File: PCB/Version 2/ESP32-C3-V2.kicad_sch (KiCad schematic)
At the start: 33 parts, among them J2 DPS_PPS_Right_Angle, J3 HCZZ0001-4, SW1 TS-1187A-B-A-B, SW2 TS-1187A-B-A-B, U1 USB-C-16P-SMD, U3 ESP32-C3, Y1 40MHz_S3240000151040

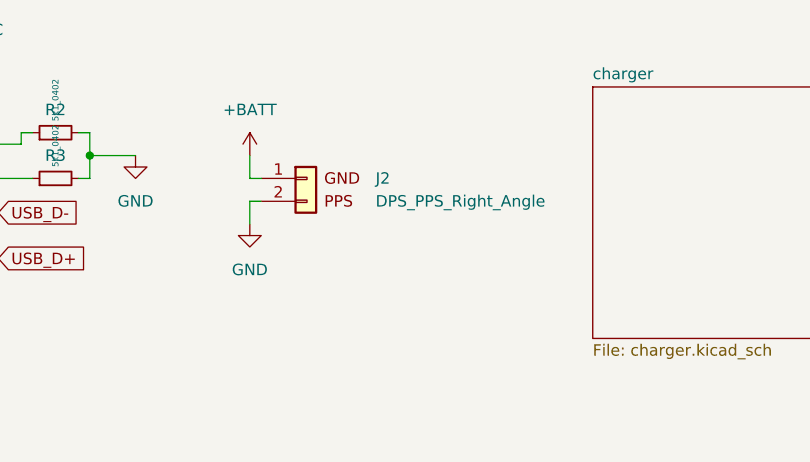
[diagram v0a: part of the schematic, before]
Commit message: update
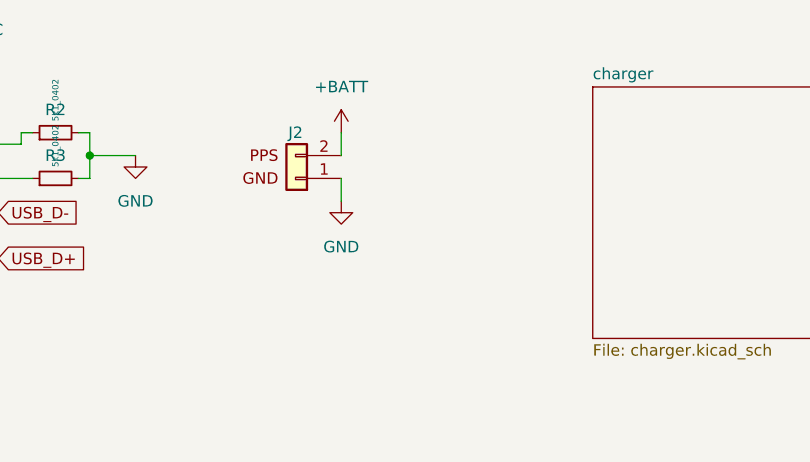
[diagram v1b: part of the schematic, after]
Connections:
- net +BATT: now also J2.2 (Pin_2); no longer J2.1 (Pin_1)
- net GND: now also J2.1 (Pin_1); no longer J2.2 (Pin_2)
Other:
- moved on the sheet: J2
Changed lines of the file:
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@@
 	(wire
 		(pts
-			(xy 76.2 34.29) (xy 74.93 34.29)
-		)
-		(stroke
-			(width 0)
-			(type default)
-		)
-	)
-	(wire
-		(pts
 			(xy 132.08 135.89) (xy 133.35 135.89)
 		)
@@
 	(wire
 		(pts
-			(xy 74.93 31.75) (xy 74.93 34.29)
+			(xy 85.09 29.21) (xy 85.09 31.75)
 		)
 		(stroke
@@
 	(wire
 		(pts
-			(xy 74.93 36.83) (xy 76.2 36.83)
-		)
-		(stroke
-			(width 0)
-			(type default)
-		)
-	)
-	(wire
-		(pts
 			(xy 45.72 43.18) (xy 46.99 43.18)
 		)
@@
 	(wire
 		(pts
-			(xy 74.93 39.37) (xy 74.93 36.83)
+			(xy 85.09 36.83) (xy 85.09 34.29)
 		)
 		(stroke
@@
 	(symbol
 		(lib_id "power:GND")
-		(at 74.93 39.37 0)
+		(at 85.09 36.83 0)
 		(unit 1)
 		(exclude_from_sim no)
@@
 		(fields_autoplaced yes)
 		(property "Reference" "#PWR06"
-			(at 74.93 45.72 0)
+			(at 85.09 43.18 0)
 			(effects
 				(font
@@
 		)
 		(property "Value" "GND"
-			(at 74.93 44.45 0)
+			(at 85.09 41.91 0)
 			(effects
 				(font
@@
 		)
 		(property "Footprint" ""
-			(at 74.93 39.37 0)
+			(at 85.09 36.83 0)
 			(effects
 				(font
@@
 		)
 		(property "Datasheet" ""
-			(at 74.93 39.37 0)
+			(at 85.09 36.83 0)
 			(effects
 				(font
@@
 		)
 		(property "Description" ""
-			(at 74.93 39.37 0)
+			(at 85.09 36.83 0)
 			(effects
 				(font
@@
 	(symbol
 		(lib_id "DPS_connectors:DPS_PPS_Right_Angle")
-		(at 81.28 35.56 0)
+		(at 80.01 33.02 180)
 		(unit 1)
 		(exclude_from_sim no)
@@
 		(on_board yes)
 		(dnp no)
-		(fields_autoplaced yes)
 		(property "Reference" "J2"
-			(at 88.9 34.29 0)
+			(at 80.01 29.21 0)
 			(effects
 				(font
 					(size 1.27 1.27)
 				)
-				(justify left)
 			)
 		)
 		(property "Value" "DPS_PPS_Right_Angle"
-			(at 88.9 36.83 0)
+			(at 72.39 28.194 0)
 			(effects
 				(font
 					(size 1.27 1.27)
 				)
-				(justify left)
+				(hide yes)
 			)
 		)
 		(property "Footprint" "Connector_JST:JST_PH_S2B-PH-K_1x02_P2.00mm_Horizontal"
-			(at 81.28 36.83 0)
+			(at 80.01 31.75 0)
 			(effects
 				(font
@@
 		)
 		(property "Datasheet" "https://datasheet.lcsc.com/lcsc/2303231100_SHOU-HAN-2-0mm-2P-WZ_C5368738.pdf"
-			(at 81.28 36.83 0)
+			(at 80.01 31.75 0)
 			(effects
 				(font
@@
 		)
 		(property "Description" ""
-			(at 81.28 35.56 0)
+			(at 80.01 33.02 0)
 			(effects
 				(font
@@
 		)
 		(property "LCSC" "C7465576"
-			(at 81.28 36.83 0)
+			(at 80.01 31.75 0)
 			(effects
 				(font
@@
 	(symbol
 		(lib_id "power:+BATT")
-		(at 74.93 31.75 0)
+		(at 85.09 29.21 0)
 		(unit 1)
 		(exclude_from_sim no)
@@
 		(fields_autoplaced yes)
 		(property "Reference" "#PWR010"
-			(at 74.93 35.56 0)
+			(at 85.09 33.02 0)
 			(effects
 				(font
@@
 		)
 		(property "Value" "+BATT"
-			(at 74.93 26.67 0)
+			(at 85.09 24.13 0)
 			(effects
 				(font
@@
 		)
 		(property "Footprint" ""
-			(at 74.93 31.75 0)
+			(at 85.09 29.21 0)
 			(effects
 				(font
@@
 		)
 		(property "Datasheet" ""
-			(at 74.93 31.75 0)
+			(at 85.09 29.21 0)
 			(effects
 				(font
@@
 		)
 		(property "Description" ""
-			(at 74.93 31.75 0)
+			(at 85.09 29.21 0)
 			(effects
 				(font

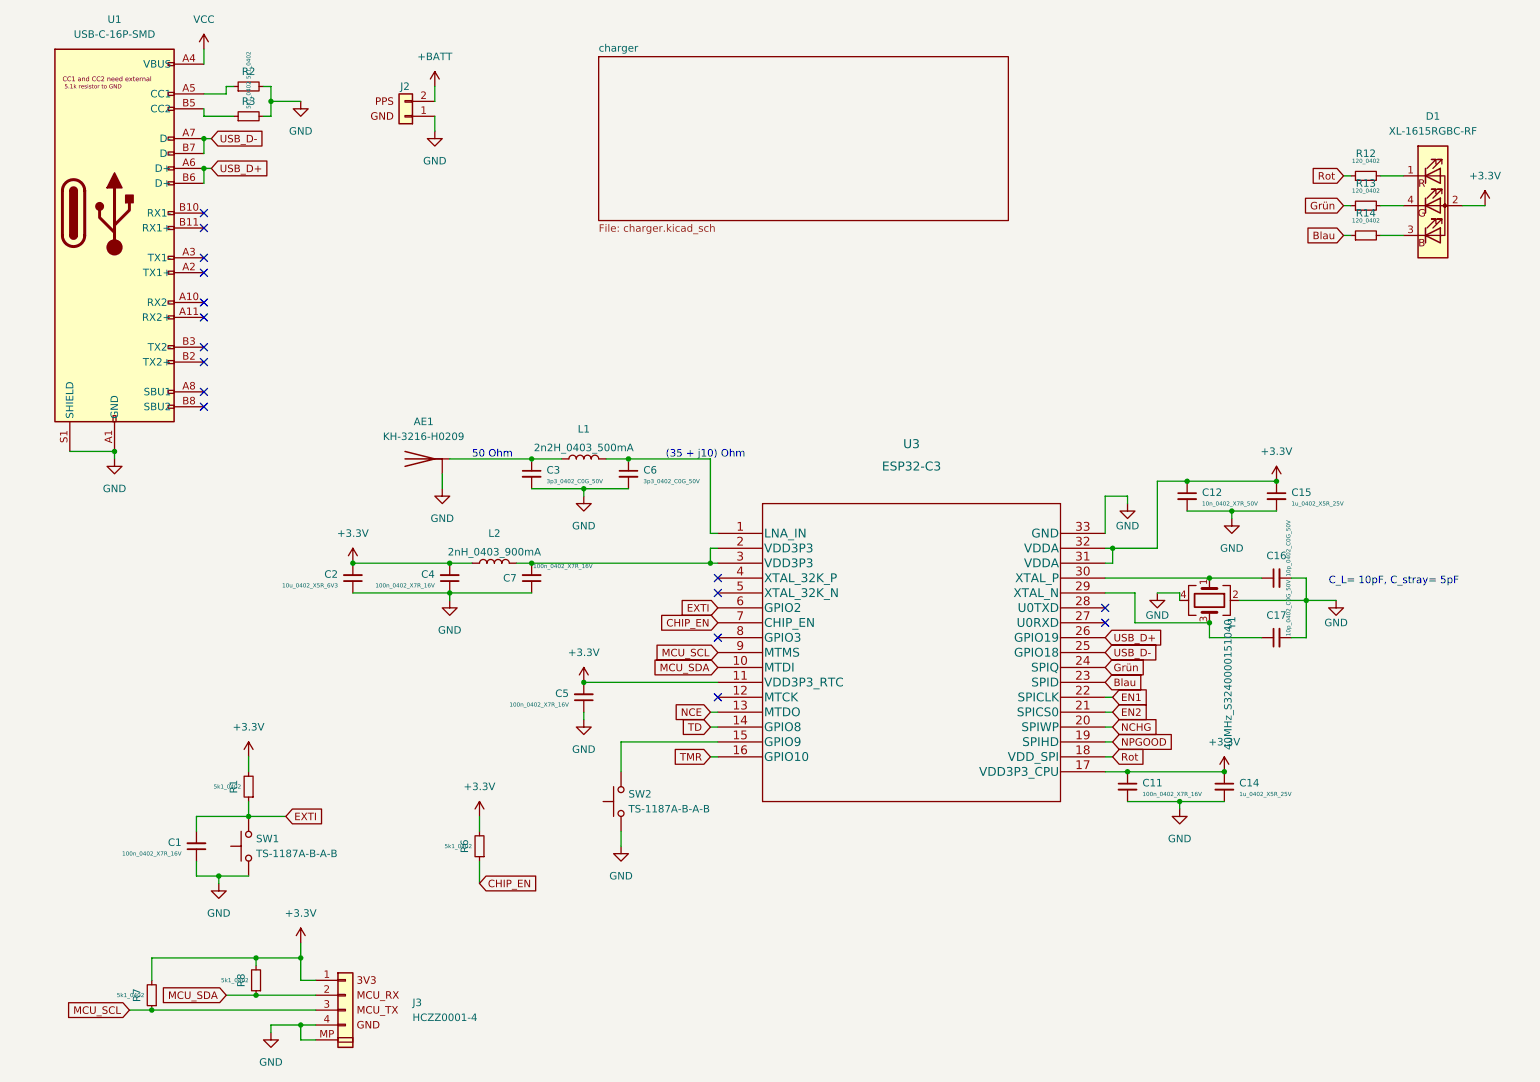
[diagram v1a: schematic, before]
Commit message: Working on Version 2
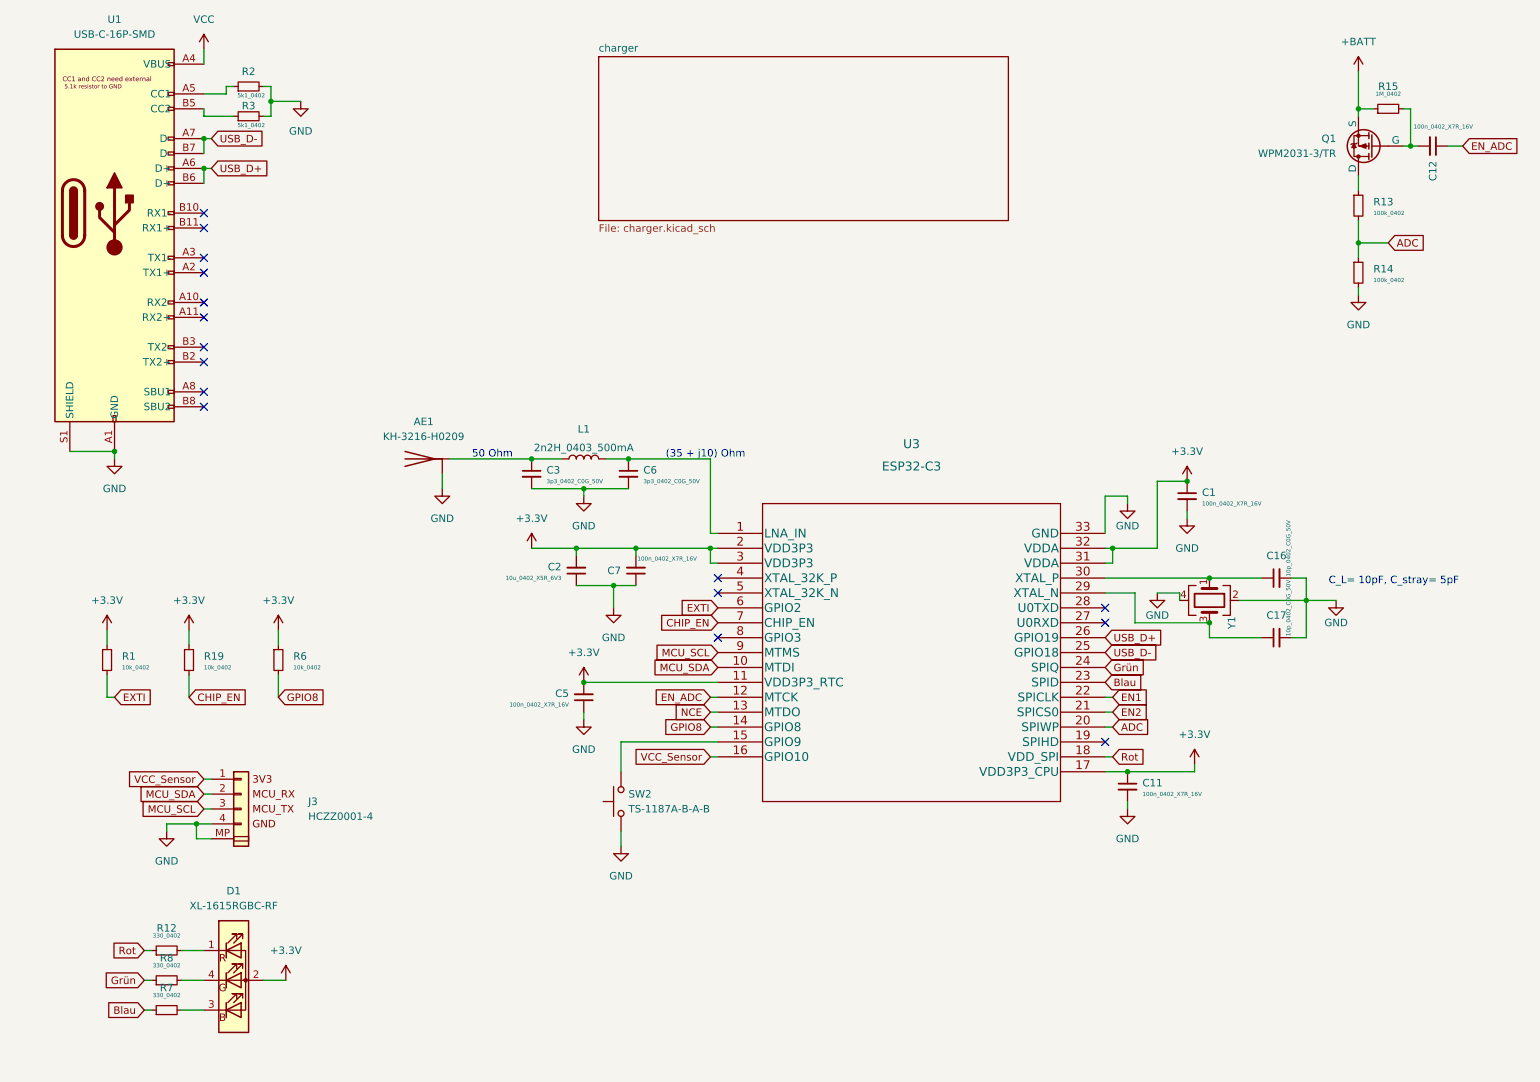
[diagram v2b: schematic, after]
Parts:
- removed C12: 10n_0402_X7R_50V, Capacitor_SMD:C_0402_1005Metric, symbol capacitor_smd_standard:10n_0402_X7R_50V
- removed C14, C15: 1u_0402_X5R_25V, Capacitor_SMD:C_0402_1005Metric, symbol capacitor_smd_standard:1u_0402_X5R_25V
- removed C4: 100n_0402_X7R_16V, Capacitor_SMD:C_0402_1005Metric, symbol capacitor_smd_standard:100n_0402_X7R_16V
- removed J2: DPS_PPS_Right_Angle, Connector_JST:JST_PH_S2B-PH-K_1x02_P2.00mm_Horizontal, symbol DPS_connectors:DPS_PPS_Right_Angle
- removed L2: 2nH_0403_900mA, Resistor_SMD:R_0402_1005Metric, symbol ESP32-C3_Bib:2nH_0403_900mA
- removed R1, R6, R7, R8: 5k1_0402, Resistor_SMD:R_0402_1005Metric, symbol resistor_smd_standard:5k1_0402
- removed R12, R13, R14: 120_0402, Resistor_SMD:R_0402_1005Metric, symbol resistor_smd_standard:120_0402
- removed SW1: TS-1187A-B-A-B, switch:SW_SPST_TL3305B, symbol 1_switch:TS-1187A-B-A-B
- added C12: 100n_0402_X7R_16V, Capacitor_SMD:C_0402_1005Metric, symbol capacitor_smd_standard:100n_0402_X7R_16V
- added Q1: WPM2031-3/TR, Package_TO_SOT_SMD:SOT-723, symbol Lil-Lib:PMOS
- added R1, R19, R6: 10k_0402, Resistor_SMD:R_0402_1005Metric, symbol resistor_smd_standard:10k_0402
- added R12, R7, R8: 330_0402, Resistor_SMD:R_0402_1005Metric, symbol resistor_smd_standard:330_0402
- added R13, R14: 100k_0402, Resistor_SMD:R_0402_1005Metric, symbol resistor_smd_standard:100k_0402
- added R15: 1M_0402, Resistor_SMD:R_0402_1005Metric, symbol resistor_smd_standard:1M_0402
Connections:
- net +3.3V: now also C1.1, C7.2, U3.2 (VDD3P3), U3.3 (VDD3P3), R1.1, R19.1, R6.1; no longer J3.1 (Pin_1)
- net +BATT: now also Q1.2 (S), R15.1
- net Blau: now also R7.1
- net CHIP_EN: now also R19.2
- net EXTI: now also R1.2; no longer C1.2
- net GND: now also C1.2, R14.2; no longer C1.1
- net Grün: now also R8.1
- net Rot: now also R12.1
- net at D1.1 (RK): now also R12.2
- net at D1.3 (BK): now also R7.2
- net at D1.4 (GK): now also R8.2
- net EN_ADC: now reaches U3.12 (MTCK)
- net EN_ADC: now also C12.1
- net NCHG renamed ADC
- net ADC: now also R13.2, R14.1
- net NPGOOD: no longer names the net of U3.19 (SPIHD)
- net TD renamed GPIO8
- net GPIO8: now also R6.2
- net TMR renamed VCC_Sensor
- net VCC_Sensor: now also J3.1 (Pin_1)
- new net: C12.2, Q1.1 (G), R15.2
- new net: Q1.3 (D), R13.1
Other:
- moved on the sheet: C2, C7, D1

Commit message: Version 2
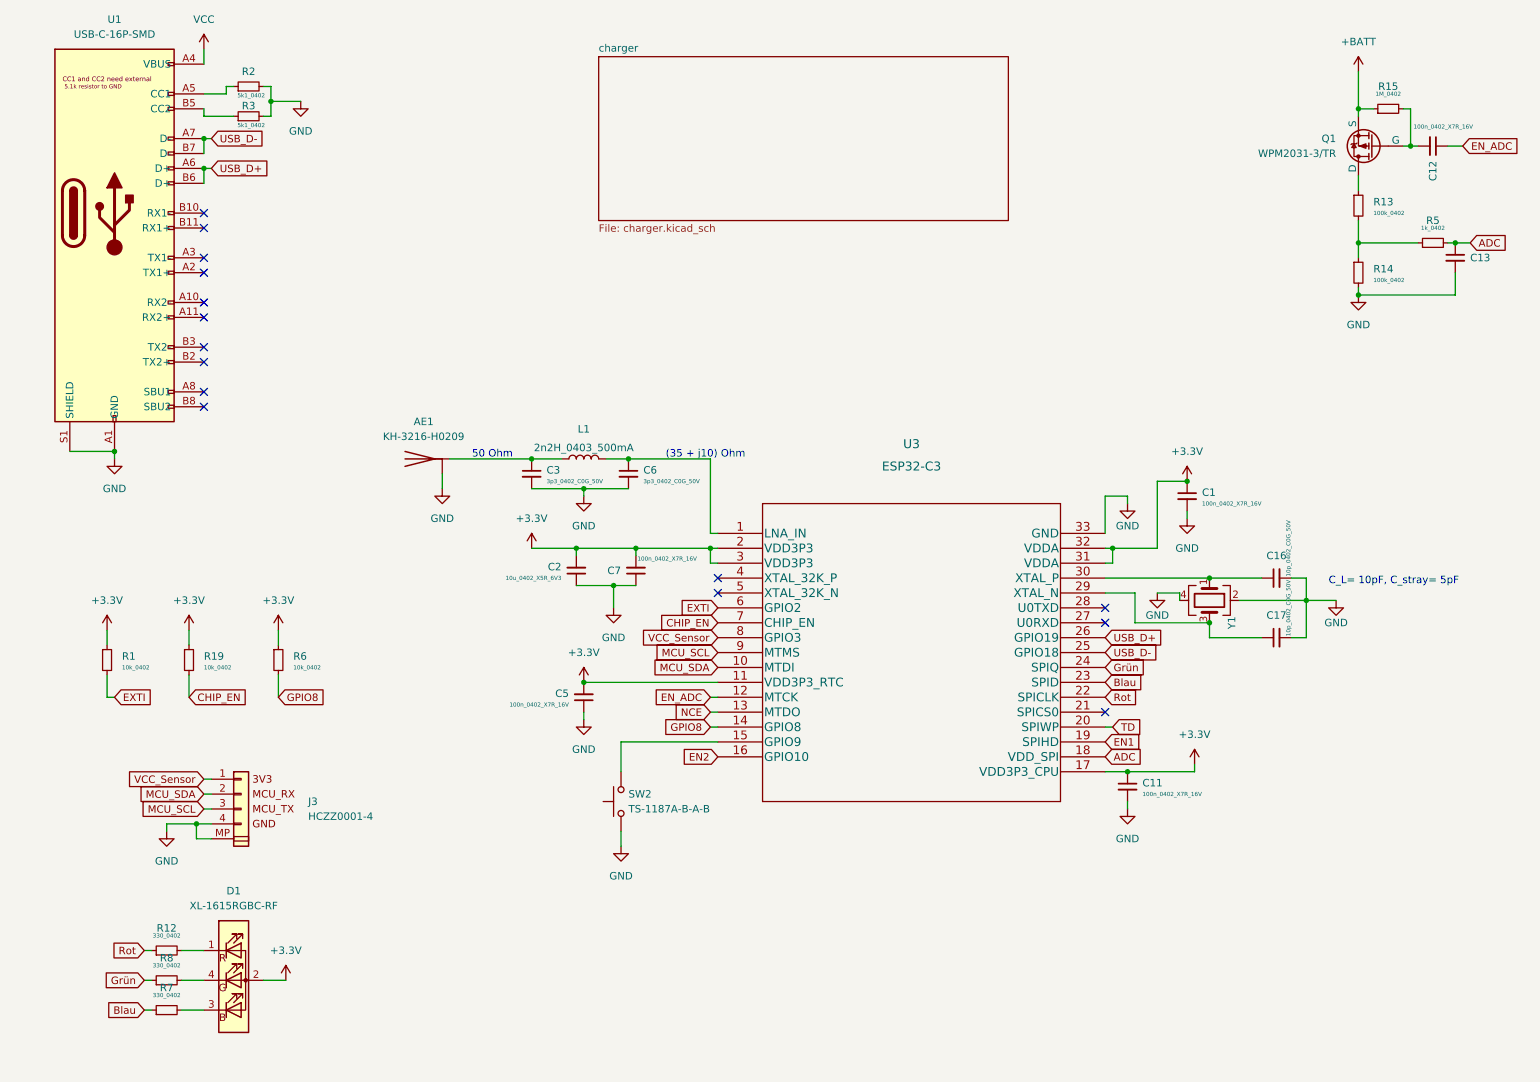
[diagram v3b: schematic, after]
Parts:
- added C13: 100n_0402_X7R_16V, Capacitor_SMD:C_0402_1005Metric, symbol capacitor_smd_standard:100n_0402_X7R_16V
- added R5: 1k_0402, Resistor_SMD:R_0402_1005Metric, symbol resistor_smd_standard:1k_0402
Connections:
- net ADC: now also U3.18 (VDD_SPI), C13.1, R5.2; no longer R13.2, R14.1, U3.20 (SPIWP)
- net EN1: now also U3.19 (SPIHD); no longer U3.22 (SPICLK)
- net EN2: now also U3.16 (GPIO10); no longer U3.21 (SPICS0)
- net GND: now also C13.2
- net Rot: now also U3.22 (SPICLK); no longer U3.18 (VDD_SPI)
- net VCC_Sensor: now also U3.8 (GPIO3); no longer U3.16 (GPIO10)
- new net: R13.2, R14.1, R5.1
- new net TD: U3.20 (SPIWP)
- no-connect marks 16 -> 15

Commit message: V2 für Kontrolle fertig
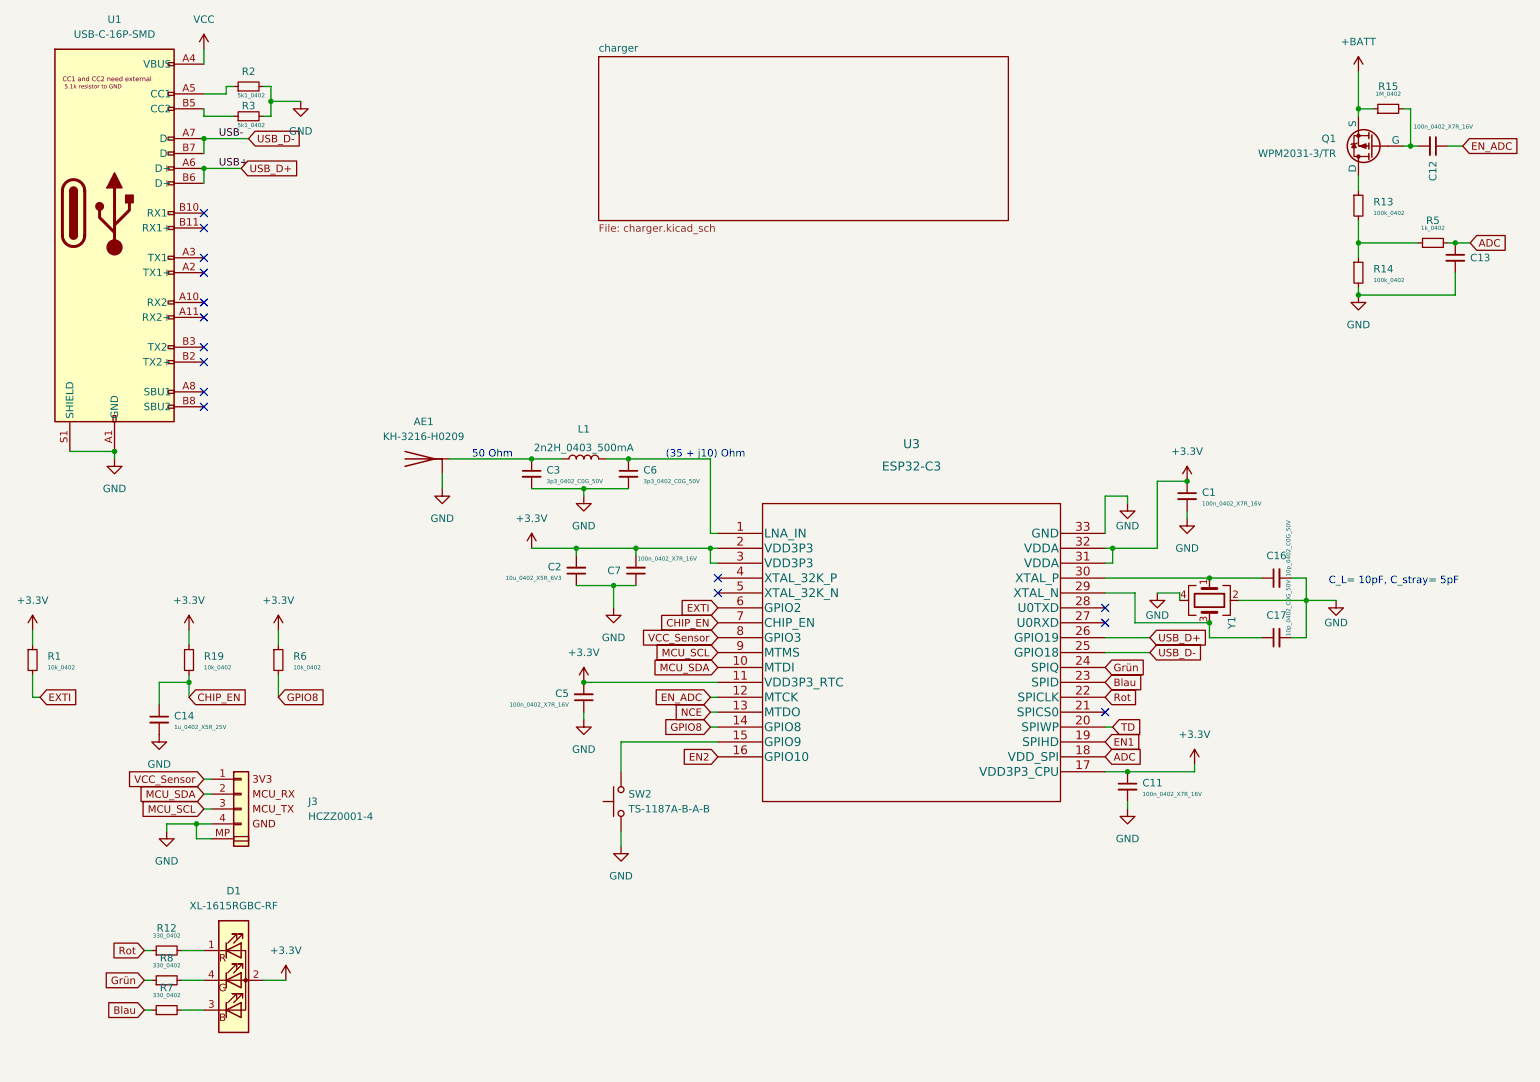
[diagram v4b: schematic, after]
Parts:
- added C14: 1u_0402_X5R_25V, Capacitor_SMD:C_0402_1005Metric, symbol capacitor_smd_standard:1u_0402_X5R_25V
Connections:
- net CHIP_EN: now also C14.1
- net GND: now also C14.2
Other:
- moved on the sheet: R1
